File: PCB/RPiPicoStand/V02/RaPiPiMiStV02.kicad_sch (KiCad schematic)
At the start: 24 parts, among them J1 Conn_01x04_Pin, J2 Conn_01x04_Pin, J3 Conn_02x20_Counter_Clockwise, J4 Conn_01x04_Pin, J5 Conn_01x02_Pin, SW1 SW_DIP_x03, SW2 SW_DIP_x03, SW3 SW_DIP_x03

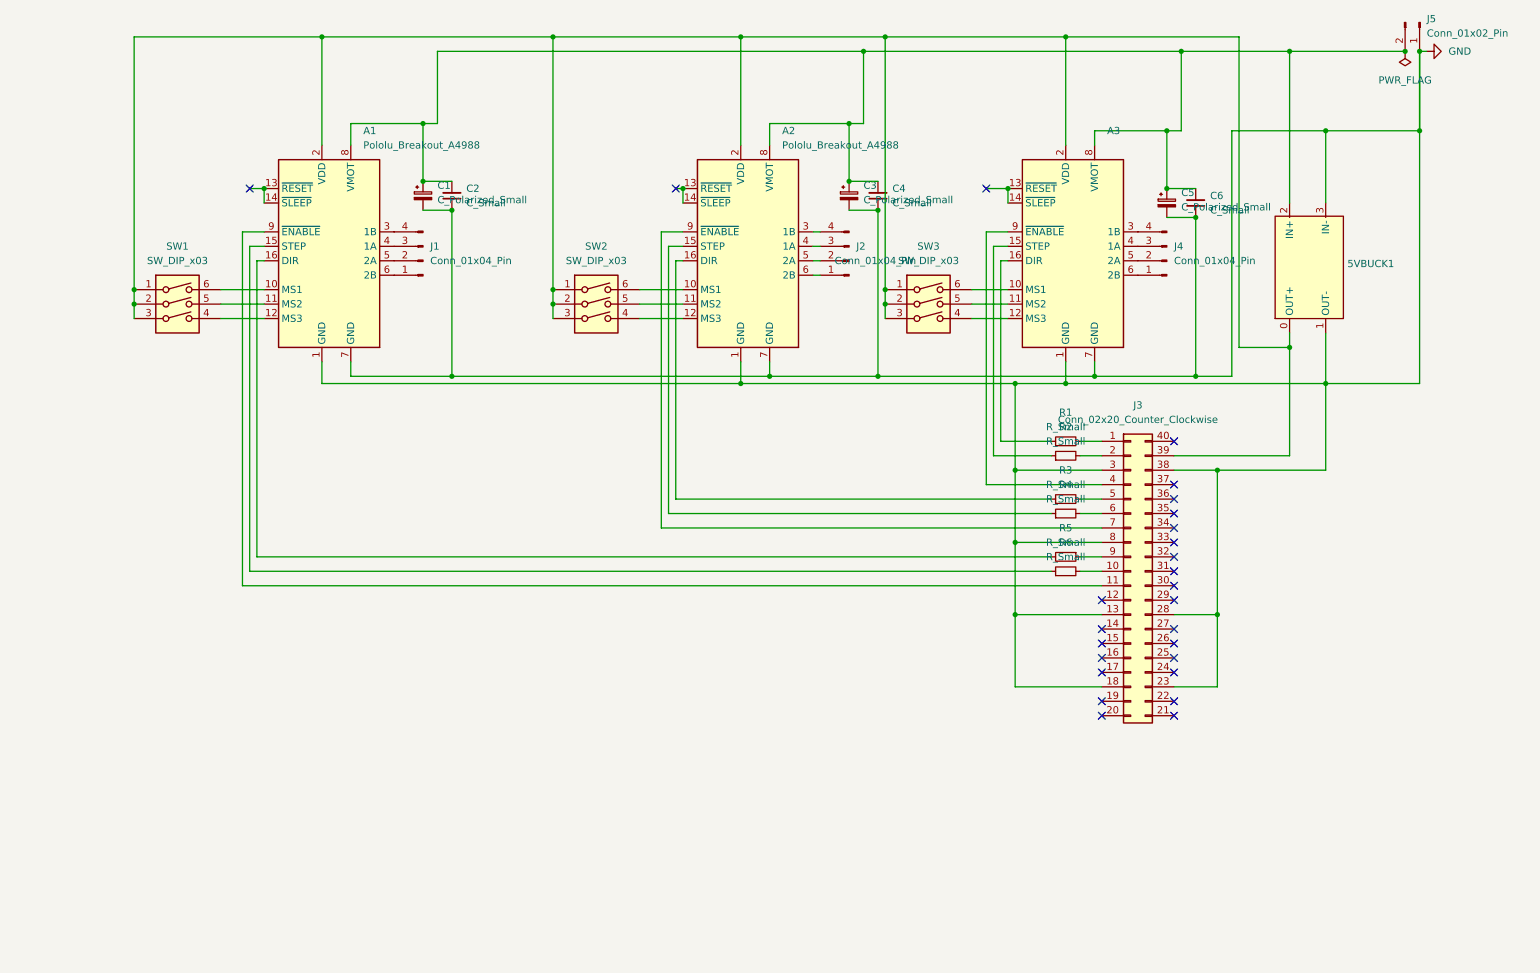
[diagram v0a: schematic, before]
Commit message: add V2 kicad project
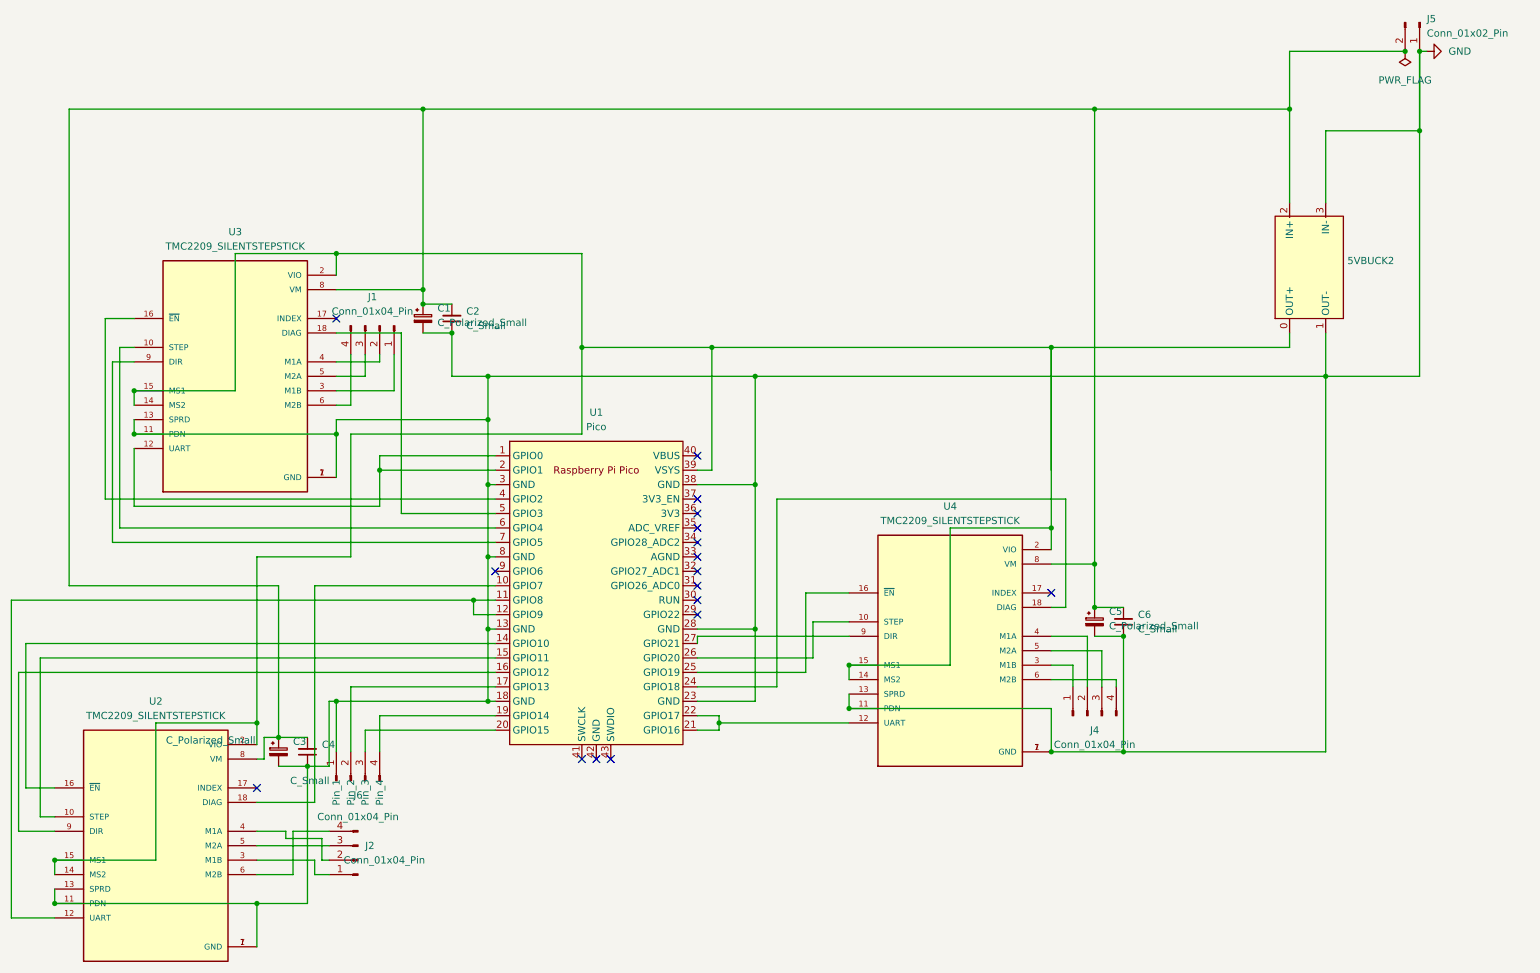
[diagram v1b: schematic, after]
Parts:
- removed 5VBUCK1: ~, Library:BUCK Converter 5-30V 5V 3A smd, symbol Driver_Motor:BUCK_CONVERTER_5-30V_to_5V_3A
- removed A1, A2, A3: Pololu_Breakout_A4988, Module:Pololu_Breakout-16_15.2x20.3mm, symbol Driver_Motor:Pololu_Breakout_A4988
- removed J3: Conn_02x20_Counter_Clockwise, Connector:DIP-40_709_ELL socket W18Pins W21, symbol Connector_Generic:Conn_02x20_Counter_Clockwise
- removed R1, R2, R3, R4, R5, R6: R_Small, Resistor_THT:R_Axial_DIN0207_L6.3mm_D2.5mm_P10.16mm_Horizontal, symbol Device:R_Small
- removed SW1, SW2, SW3: SW_DIP_x03, Button_Switch_THT:SW_DIP_SPSTx03_Slide_9.78x9.8mm_W7.62mm_P2.54mm, symbol Switch:SW_DIP_x03
- added 5VBUCK2: ~, RaPiPiMiSt:BUCK Converter 5-30V 5V 3A smd, symbol RaPiPiMiSt:BUCK_CONVERTER_5-30V_to_5V_3A
- added J6: Conn_01x04_Pin, Connector_PinSocket_2.54mm:PinSocket_1x04_P2.54mm_Vertical, symbol Connector:Conn_01x04_Pin
- added U1: Pico, MCU_RaspberryPi_and_Boards:RPi_Pico_SMD_TH, symbol MCU_RaspberryPi_and_Boards:Pico
- added U2, U3, U4: TMC2209_SILENTSTEPSTICK, RaPiPiMiSt:MODULE_TMC2209_SILENTSTEPSTICK, symbol RaPiPiMiSt:TMC2209_SILENTSTEPSTICK
- C1, C3, C5: footprint Capacitor_THT:CP_Radial_D7.5mm_P2.50mm -> Capacitor_SMD:CP_Elec_6.3x7.7
- C2, C4, C6: footprint Capacitor_THT:C_Disc_D6.0mm_W2.5mm_P5.00mm -> Capacitor_SMD:C_0603_1608Metric
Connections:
- net GND: now also 5VBUCK2.1 (OUT-), 5VBUCK2.3 (IN-), J6.1 (Pin_1), U1.13 (GND), U1.18 (GND), U1.23 (GND), U1.28 (GND), U1.3 (GND), U1.38 (GND), U1.8 (GND), U2.1 (GND), U2.11 (PDN), U2.13 (SPRD), U2.7 (GND), U3.1 (GND), U3.11 (PDN), U3.13 (SPRD), U3.7 (GND), U4.1 (GND), U4.11 (PDN), U4.13 (SPRD), U4.7 (GND)
- net at C1.1, C2.2, C3.1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: now also 5VBUCK2.2 (IN+), U2.8 (VM), U3.8 (VM), U4.8 (VM)
- net at J2.1 (Pin_1): now also U2.3 (M1B)
- net at J2.2 (Pin_2): now also U2.4 (M1A)
- net at J2.3 (Pin_3): now also U2.5 (M2A)
- net at J2.4 (Pin_4): now also U2.6 (M2B)
- net at J1.1 (Pin_1): now also U3.3 (M1B)
- net at J1.2 (Pin_2): now also U3.4 (M1A)
- net at J1.3 (Pin_3): now also U3.5 (M2A)
- net at J1.4 (Pin_4): now also U3.6 (M2B)
- net at J4.4 (Pin_4): now also U4.6 (M2B)
- net at J4.3 (Pin_3): now also U4.5 (M2A)
- net at J4.2 (Pin_2): now also U4.4 (M1A)
- net at J4.1 (Pin_1): now also U4.3 (M1B)
- new net: J6.2 (Pin_2), U1.17 (GPIO13)
- new net: J6.3 (Pin_3), U1.20 (GPIO15)
- new net: J6.4 (Pin_4), U1.19 (GPIO14)
- new net: U1.6 (GPIO4), U3.10 (STEP)
- new net: U1.1 (GPIO0), U1.2 (GPIO1), U3.12 (UART)
- new net: 5VBUCK2.0 (OUT+), U1.39 (VSYS), U2.14 (MS2), U2.15 (MS1), U2.2 (VIO), U3.14 (MS2), U3.15 (MS1), U3.2 (VIO), U4.14 (MS2), U4.15 (MS1), U4.2 (VIO)
- new net: U1.4 (GPIO2), U3.16 (~{EN})
- new net: U1.5 (GPIO3), U3.18 (DIAG)
- new net: U1.7 (GPIO5), U3.9 (DIR)
- new net: U1.26 (GPIO20), U4.10 (STEP)
- new net: U1.21 (GPIO16), U1.22 (GPIO17), U4.12 (UART)
- new net: U1.25 (GPIO19), U4.16 (~{EN})
- new net: U1.24 (GPIO18), U4.18 (DIAG)
- new net: U1.27 (GPIO21), U4.9 (DIR)
- new net: U1.10 (GPIO7), U2.18 (DIAG)
- new net: U1.11 (GPIO8), U1.12 (GPIO9), U2.12 (UART)
- new net: U1.14 (GPIO10), U2.16 (~{EN})
- new net: U1.15 (GPIO11), U2.10 (STEP)
- new net: U1.16 (GPIO12), U2.9 (DIR)
- no-connect marks 26 -> 17
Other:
- moved on the sheet: C1, C2, C3, C4, C5, C6, J1, J2, J4
